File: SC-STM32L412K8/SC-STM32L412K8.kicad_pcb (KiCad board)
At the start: 2 copper layers, 31.6 x 15.1 mm, 70 parts, among them J1 usb, J10 PWM, J11 Vibro, J12 +3v, J13 +vibro, J2 +29.6 SiPM, J3 TxD, J4 RxD, J5 SWDIO, J6 SWCLK, J7 +BAT, J8 SiPM-, J9 BT Status, Q1 IRLML5203, Q2 KT235, Q3 KT235, SW1 power, U1 LP2985-3.0, U2 LM2733YMF, U3 LTC4054ES5, U4 LMV7239M5, U5 MCP1700-3002E

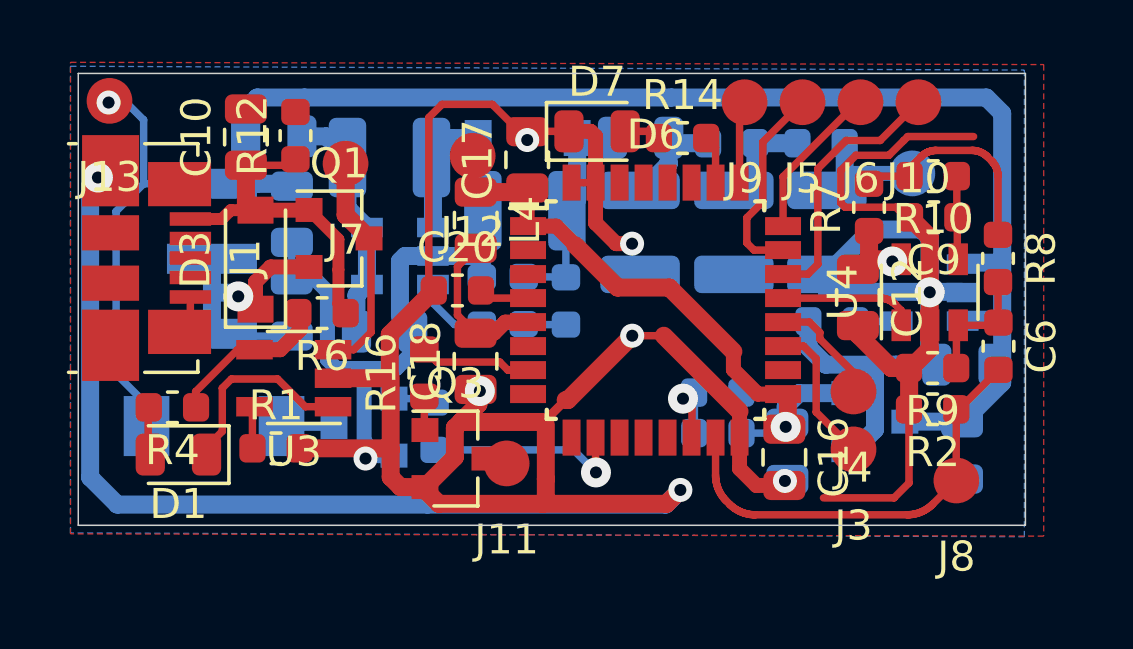
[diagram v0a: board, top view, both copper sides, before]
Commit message: modified:   SC-STM32L412K8/SC-STM32L412K8.kicad_pcb 	modified:   SC-STM32L412K8/SC-STM32L412K8.kicad_pcb-bak 	modified:   SC-STM32L412K8/SC-STM32L412K8.net 	modified:   SC-STM32L412K8/SC-STM32L412K8.sch 	modified:   SC-STM32L412K8/SC-STM32L412K8.sch-bak
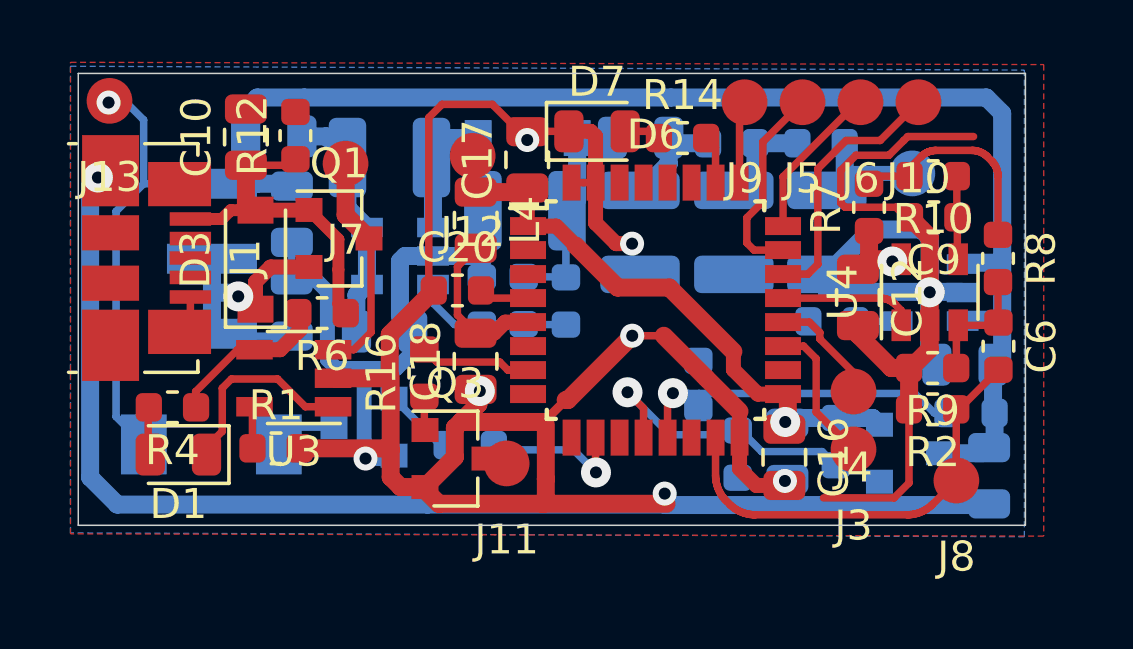
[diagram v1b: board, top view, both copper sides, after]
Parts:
- added R19: X, Resistor_SMD:R_0603_1608Metric, B.Cu at (56.9, 94.7)
- added R20: X, Resistor_SMD:R_0603_1608Metric, B.Cu at (47.8, 93.8)
- moved R17 3.94 mm to (52.4, 95.7), turned to 90 degrees
- moved R18 2.16 mm to (49.1, 96.1), turned to 90 degrees
- moved U5 1.56 mm to (54.8, 96.1)
- moved R15 1.35 mm to (40.2, 95.8), turned to 0 degrees
- moved C15 1.23 mm to (57.5, 96.8)
- moved BZ1 0.62 mm to (31.6, 95.8)
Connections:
- D6 pad 12: (no net) -> tm
- D6 pad 13: (no net) -> bl
- D6 pad 14: tm -> (no net)
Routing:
- net bl: track 0.00 -> 11.3 mm, vias 0 -> 1
- net tm: track 2.59 -> 9.80 mm
- net Buzer: track 6.86 -> 4.95 mm
- net GND: track 161.9 -> 162.9 mm
- net Net-(Q2-Pad1): track 1.52 -> 2.40 mm
- net +BATT: track 61.1 -> 61.9 mm

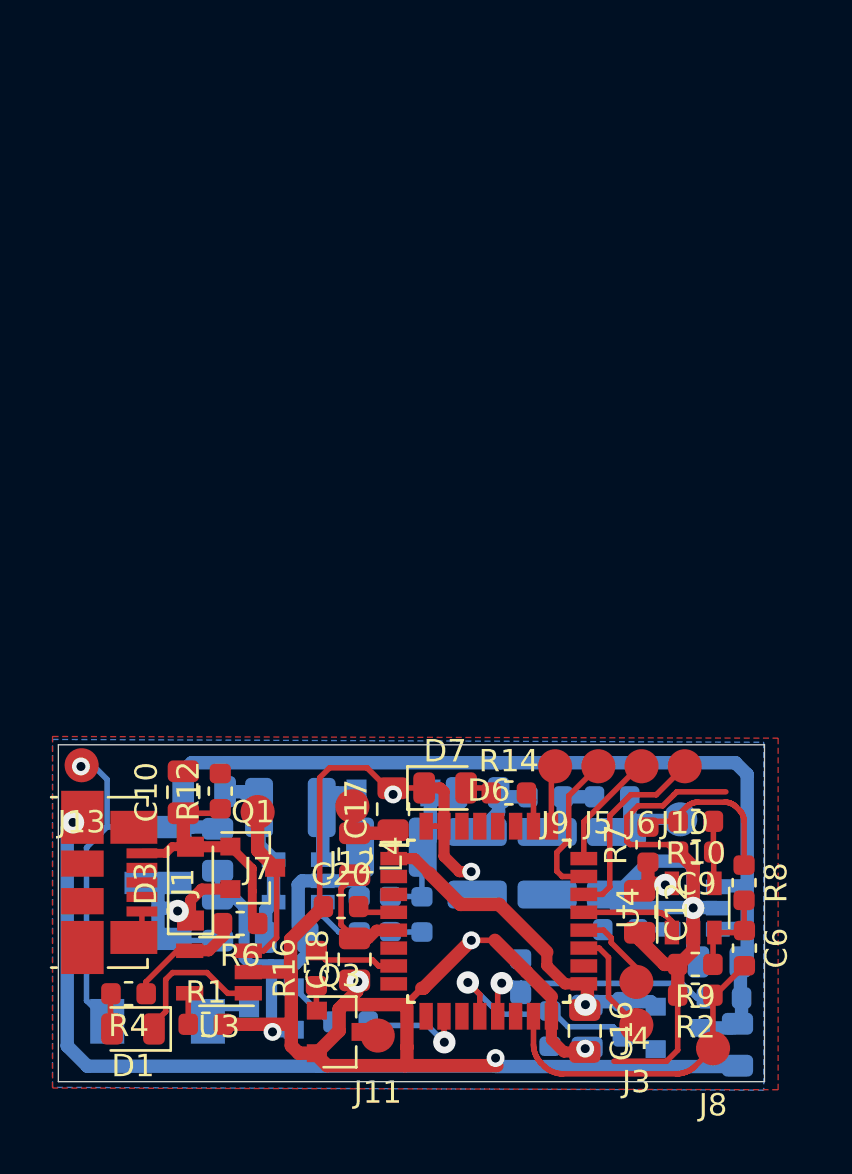
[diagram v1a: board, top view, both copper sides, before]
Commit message: изменено:      SC-STM32L412K8/SC-STM32L412K8-cache.lib 	изменено:      SC-STM32L412K8/SC-STM32L412K8.kicad_pcb 	изменено:      SC-STM32L412K8/SC-STM32L412K8.kicad_pcb-bak 	изменено:      SC-STM32L412K8/SC-STM32L412K8.sch 	изменено:      SC-STM32L412K8/SC-STM32L412K8.sch-bak 	SC-STM32L412K8/SC-STM32L412K8-rescue.dcm 	SC-STM32L412K8/SC-STM32L412K8-rescue.lib
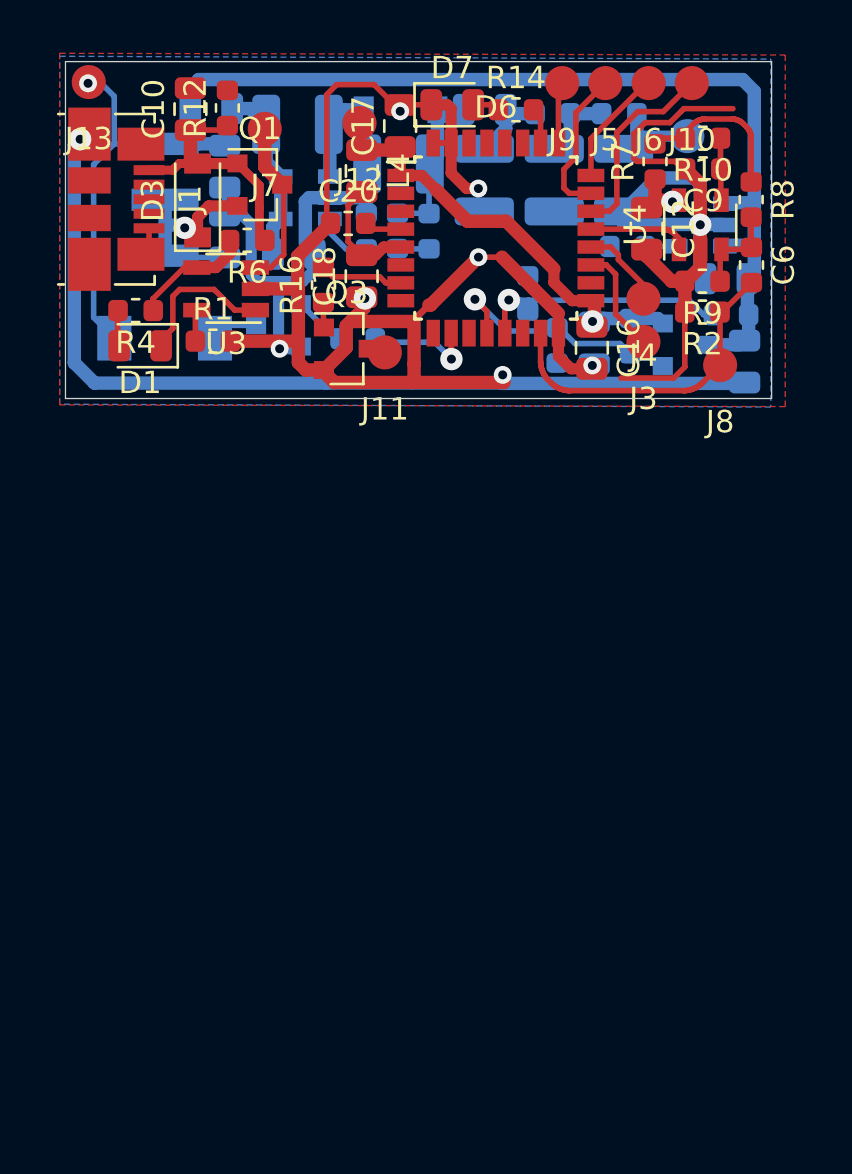
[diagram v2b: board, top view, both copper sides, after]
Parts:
- moved C15 30.5 mm to (57.8, 66.3)
- moved C19 30.5 mm to (51.1, 65.5)
- moved C20 30.5 mm to (40.1, 60.1)
- moved C9 30.5 mm to (56.0, 57.7)
- moved D1 30.5 mm to (30.8, 65.6)
- moved J11 30.5 mm to (41.7, 65.9)
- moved J3 30.5 mm to (53.3, 65.4)
- moved L1 30.5 mm to (34.0, 55.0)
- moved Q2 30.5 mm to (37.0, 64.7)
- moved Q3 30.5 mm to (40.0, 65.7)
- moved R1 30.5 mm to (34.0, 65.4)
- moved R11 30.5 mm to (49.2, 55.2)
- moved R13 30.5 mm to (52.2, 55.2)
- moved R15 30.5 mm to (40.5, 65.3)
- moved R8 30.5 mm to (58.1, 59.0)
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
